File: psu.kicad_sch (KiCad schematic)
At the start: 21 parts, among them U5 TPS7A8001DRBR, U6 TPS7A8001DRBR

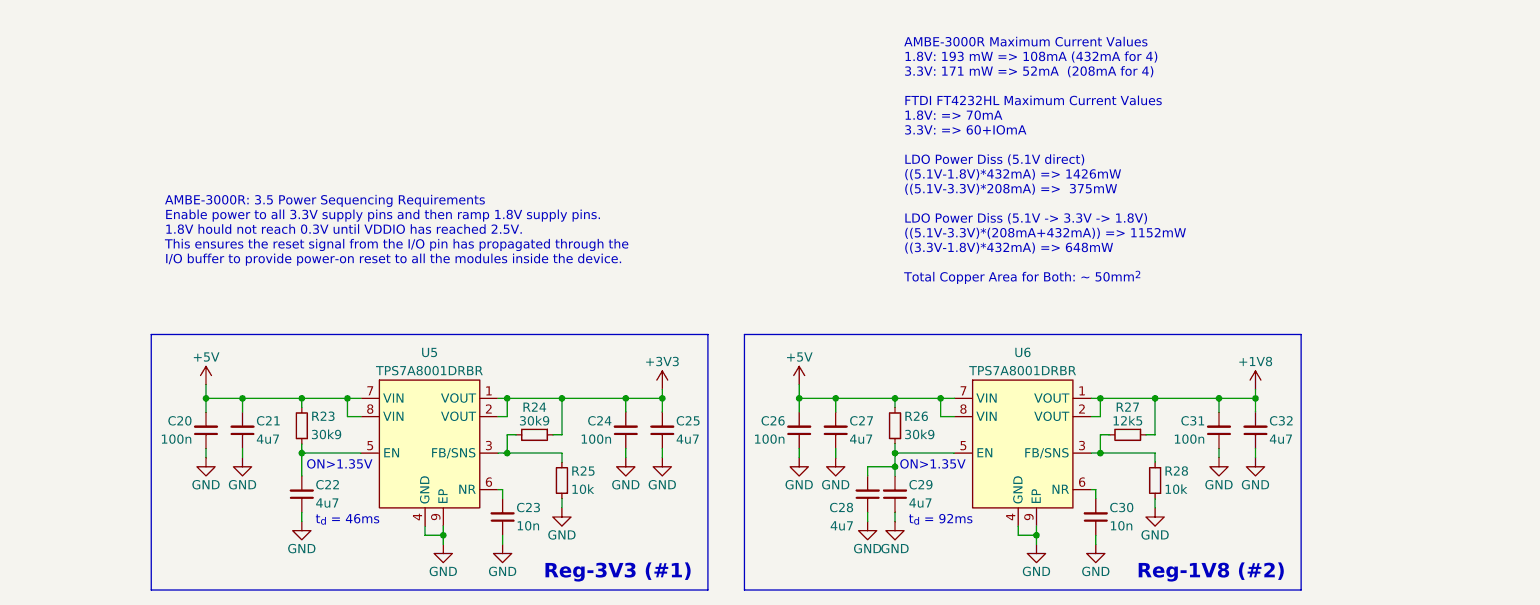
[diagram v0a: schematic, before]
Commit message: Final updates before manufacture of V1.00
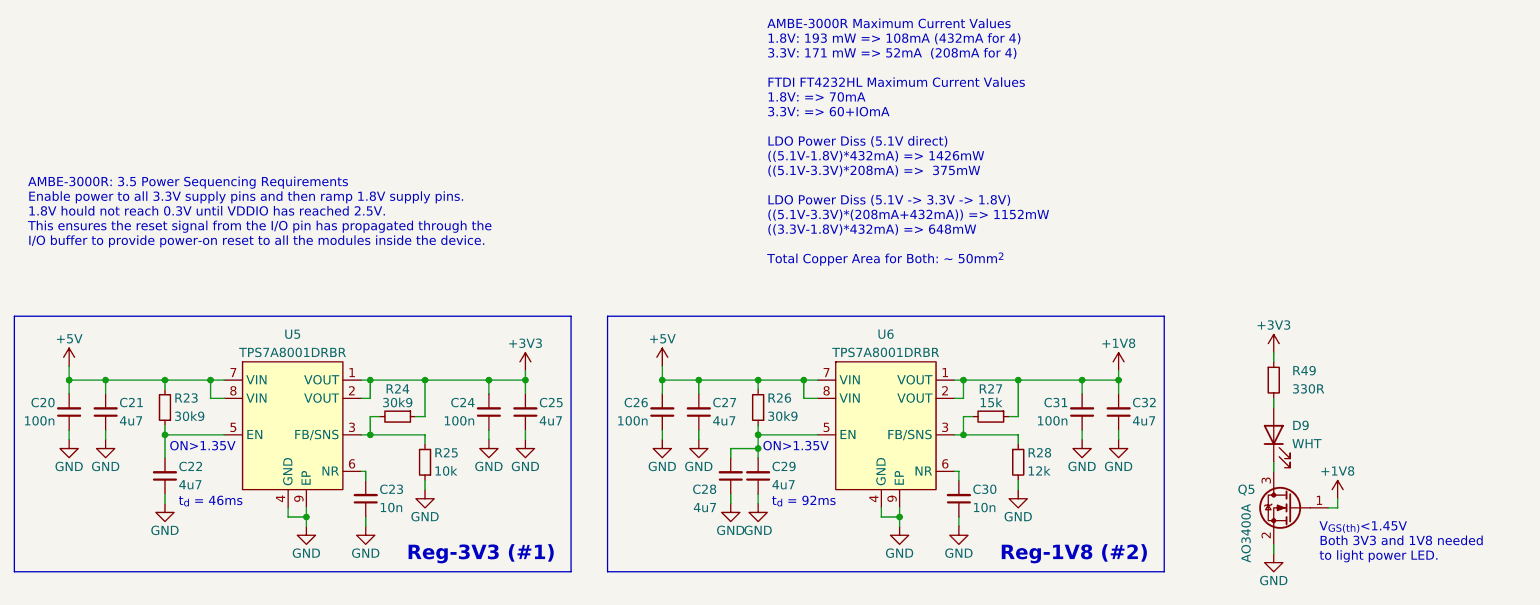
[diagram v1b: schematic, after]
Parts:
- added D9: WHT, LED_SMD:LED_0603_1608Metric, symbol Device:LED
- added Q5: AO3400A, Package_TO_SOT_SMD:SOT-23, symbol Transistor_FET:AO3400A
- added R49: 330R, Resistor_SMD:R_0603_1608Metric, symbol Device:R_Small
- C20, C24, C26, C31: LCSC (none) -> C14663
- C21, C22, C25, C27, C28, C29, C32: LCSC (none) -> C19666
- C23, C30: LCSC (none) -> C57112
- R23, R24, R26: LCSC (none) -> C217957
- R25: LCSC (none) -> C25804
- R27: value 12k5 -> 15k; LCSC (none) -> C22809
- R28: value 10k -> 12k; LCSC (none) -> C22790
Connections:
- net +1V8: now also Q5.1 (G)
- net +3V3: now also R49.1
- net GND: now also R28.2, Q5.2 (S); no longer R28.1
- net at R27.2, U6.3 (FB/SNS): now also R28.1; no longer R28.2
- new net: D9.1 (K), Q5.3 (D)
- new net: D9.2 (A), R49.2
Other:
- note added: "V_{GS(th)}<1.45V Both 3V3 and 1V8 needed to light power LED."
- title: Quad AMBE-3000R Board -> Quad AMBE-3000R Board (Power Supplies & Sequencing)
- moved on the sheet: C20, C21, C22, C23, C24, C25, C26, C27, C28, C29, C30, C31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
